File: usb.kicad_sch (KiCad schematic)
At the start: 5 parts, among them J13 USB-C 2.0, U9 USBLC6-2SC6

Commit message: friday changes
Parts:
- D7: DigiKey (none) -> 1655-DSS14UTR-ND
- J13: DigiKey (none) -> 2073-USB4085-GF-ATR-ND
- R15, R16: DigiKey (none) -> RMCF1206JT5K10TR-ND; MPN (none) -> RMCF1206JT5K10; Manufacturer (none) -> Stackpole Electronics Inc
- U9: DigiKey (none) -> 5399-USBLC6-2SC6TR-ND
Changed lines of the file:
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@@
+			)
+		)
+		(property "DigiKey" "2073-USB4085-GF-ATR-ND"
+			(at 0 0 0)
+			(effects
+				(font
+					(size 1.27 1.27)
+				)
+				(hide yes)
 			)
 		)
@@
 			)
 		)
+		(property "Manufacturer" "Stackpole Electronics Inc"
+			(at 0 0 0)
+			(effects
+				(font
+					(size 1.27 1.27)
+				)
+				(hide yes)
+			)
+		)
+		(property "MPN" "RMCF1206JT5K10"
+			(at 0 0 0)
+			(effects
+				(font
+					(size 1.27 1.27)
+				)
+				(hide yes)
+			)
+		)
+		(property "DigiKey" "RMCF1206JT5K10TR-ND"
+			(at 0 0 0)
+			(effects
+				(font
+					(size 1.27 1.27)
+				)
+				(hide yes)
+			)
+		)
 		(pin "1"
 		)
@@
 			)
 		)
+		(property "Manufacturer" "Stackpole Electronics Inc"
+			(at 0 0 0)
+			(effects
+				(font
+					(size 1.27 1.27)
+				)
+				(hide yes)
+			)
+		)
+		(property "MPN" "RMCF1206JT5K10"
+			(at 0 0 0)
+			(effects
+				(font
+					(size 1.27 1.27)
+				)
+				(hide yes)
+			)
+		)
+		(property "DigiKey" "RMCF1206JT5K10TR-ND"
+			(at 0 0 0)
+			(effects
+				(font
+					(size 1.27 1.27)
+				)
+				(hide yes)
+			)
+		)
 		(pin "1"
 		)
@@
 			)
 		)
+		(property "DigiKey" "1655-DSS14UTR-ND"
+			(at 0 0 0)
+			(effects
+				(font
+					(size 1.27 1.27)
+				)
+				(hide yes)
+			)
+		)
 		(pin "1"
 		)
@@
 				(hide yes)
 			)
+		)
+		(property "DigiKey" "5399-USBLC6-2SC6TR-ND"
+			(at 0 0 0)
+			(effects
+				(font
+					(size 1.27 1.27)
+				)
+				(hide yes)
+			)

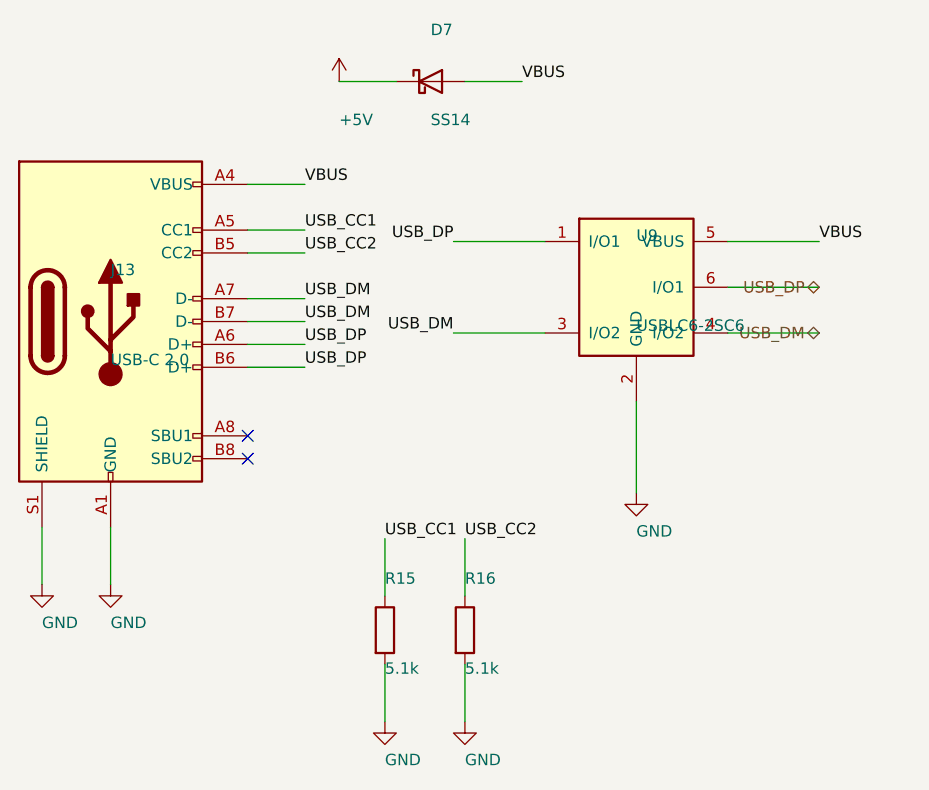
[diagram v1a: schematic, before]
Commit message: schematic updated
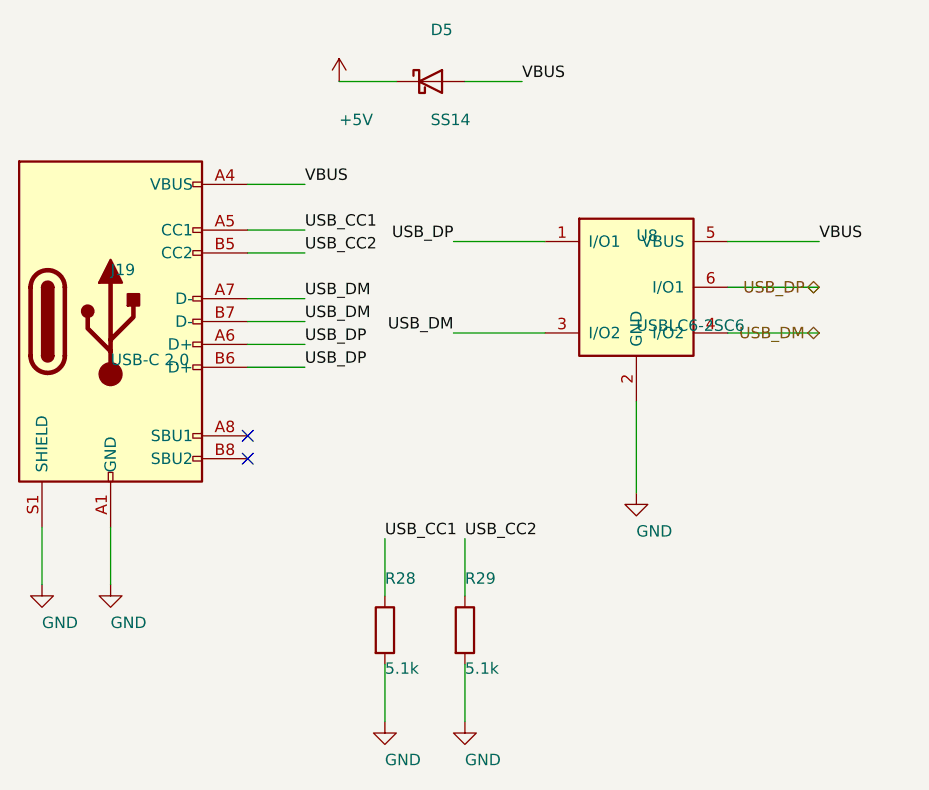
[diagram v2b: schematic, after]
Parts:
- renumbered D7 to D5, J13 to J19, R15 to R28, R16 to R29, U9 to U8
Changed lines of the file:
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@@
 		(on_board yes)
 		(dnp no)
-		(property "Reference" "J13"
+		(property "Reference" "J19"
 			(at 172.72 143.59 0)
 			(effects
@@
 			(project "controlcarreta"
 				(path "/9232987b-e923-413e-abd9-77ced6cc4c47/a9f5f58e-9f19-4b76-92d3-0178cc2d2479"
-					(reference "J13")
+					(reference "J19")
 					(unit 1)
 				)
@@
 		(on_board yes)
 		(dnp no)
-		(property "Reference" "#PWR0522"
+		(property "Reference" "#PWR0156"
 			(at 172.72 172.8 0)
 			(effects
@@
 			(project "controlcarreta"
 				(path "/9232987b-e923-413e-abd9-77ced6cc4c47/a9f5f58e-9f19-4b76-92d3-0178cc2d2479"
-					(reference "#PWR0522")
+					(reference "#PWR0156")
 					(unit 1)
 				)
@@
 		(on_board yes)
 		(dnp no)
-		(property "Reference" "#PWR0523"
+		(property "Reference" "#PWR0155"
 			(at 165.1 172.8 0)
 			(effects
@@
 			(project "controlcarreta"
 				(path "/9232987b-e923-413e-abd9-77ced6cc4c47/a9f5f58e-9f19-4b76-92d3-0178cc2d2479"
-					(reference "#PWR0523")
+					(reference "#PWR0155")
 					(unit 1)
 				)
@@
 		(on_board yes)
 		(dnp no)
-		(property "Reference" "R15"
+		(property "Reference" "R28"
 			(at 203.2 177.88 0)
 			(effects
@@
 			(project "controlcarreta"
 				(path "/9232987b-e923-413e-abd9-77ced6cc4c47/a9f5f58e-9f19-4b76-92d3-0178cc2d2479"
-					(reference "R15")
+					(reference "R28")
 					(unit 1)
 				)
@@
 		(on_board yes)
 		(dnp no)
-		(property "Reference" "#PWR0524"
+		(property "Reference" "#PWR0158"
 			(at 203.2 188.04 0)
 			(effects
@@
 			(project "controlcarreta"
 				(path "/9232987b-e923-413e-abd9-77ced6cc4c47/a9f5f58e-9f19-4b76-92d3-0178cc2d2479"
-					(reference "#PWR0524")
+					(reference "#PWR0158")
 					(unit 1)
 				)
@@
 		(on_board yes)
 		(dnp no)
-		(property "Reference" "R16"
+		(property "Reference" "R29"
 			(at 212.09 177.88 0)
 			(effects
@@
 			(project "controlcarreta"
 				(path "/9232987b-e923-413e-abd9-77ced6cc4c47/a9f5f58e-9f19-4b76-92d3-0178cc2d2479"
-					(reference "R16")
+					(reference "R29")
 					(unit 1)
 				)
@@
 		(on_board yes)
 		(dnp no)
-		(property "Reference" "#PWR0525"
+		(property "Reference" "#PWR0159"
 			(at 212.09 188.04 0)
 			(effects
@@
 			(project "controlcarreta"
 				(path "/9232987b-e923-413e-abd9-77ced6cc4c47/a9f5f58e-9f19-4b76-92d3-0178cc2d2479"
-					(reference "#PWR0525")
+					(reference "#PWR0159")
 					(unit 1)
 				)
@@
 		(on_board yes)
 		(dnp no)
-		(property "Reference" "D7"
+		(property "Reference" "D5"
 			(at 208.28 116.92 0)
 			(effects
@@
 			(project "controlcarreta"
 				(path "/9232987b-e923-413e-abd9-77ced6cc4c47/a9f5f58e-9f19-4b76-92d3-0178cc2d2479"
-					(reference "D7")
+					(reference "D5")
 					(unit 1)
 				)
@@
 		(on_board yes)
 		(dnp no)
-		(property "Reference" "#PWR0526"
+		(property "Reference" "#PWR0157"
 			(at 198.12 116.92 0)
 			(effects
@@
 			(project "controlcarreta"
 				(path "/9232987b-e923-413e-abd9-77ced6cc4c47/a9f5f58e-9f19-4b76-92d3-0178cc2d2479"
-					(reference "#PWR0526")
+					(reference "#PWR0157")
 					(unit 1)
 				)
@@
 		(on_board yes)
 		(dnp no)
-		(property "Reference" "U9"
+		(property "Reference" "U8"
 			(at 231.14 139.78 0)
 			(effects
@@
 			(project "controlcarreta"
 				(path "/9232987b-e923-413e-abd9-77ced6cc4c47/a9f5f58e-9f19-4b76-92d3-0178cc2d2479"
-					(reference "U9")
+					(reference "U8")
 					(unit 1)
 				)
@@
 		(on_board yes)
 		(dnp no)
-		(property "Reference" "#PWR0527"
+		(property "Reference" "#PWR0160"
 			(at 231.14 162.64 0)
 			(effects
@@
 			(project "controlcarreta"
 				(path "/9232987b-e923-413e-abd9-77ced6cc4c47/a9f5f58e-9f19-4b76-92d3-0178cc2d2479"
-					(reference "#PWR0527")
-					(unit 1)
-				)
+					(reference "#PWR0160")
+					(unit 1)
+				)

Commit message: last changes in work
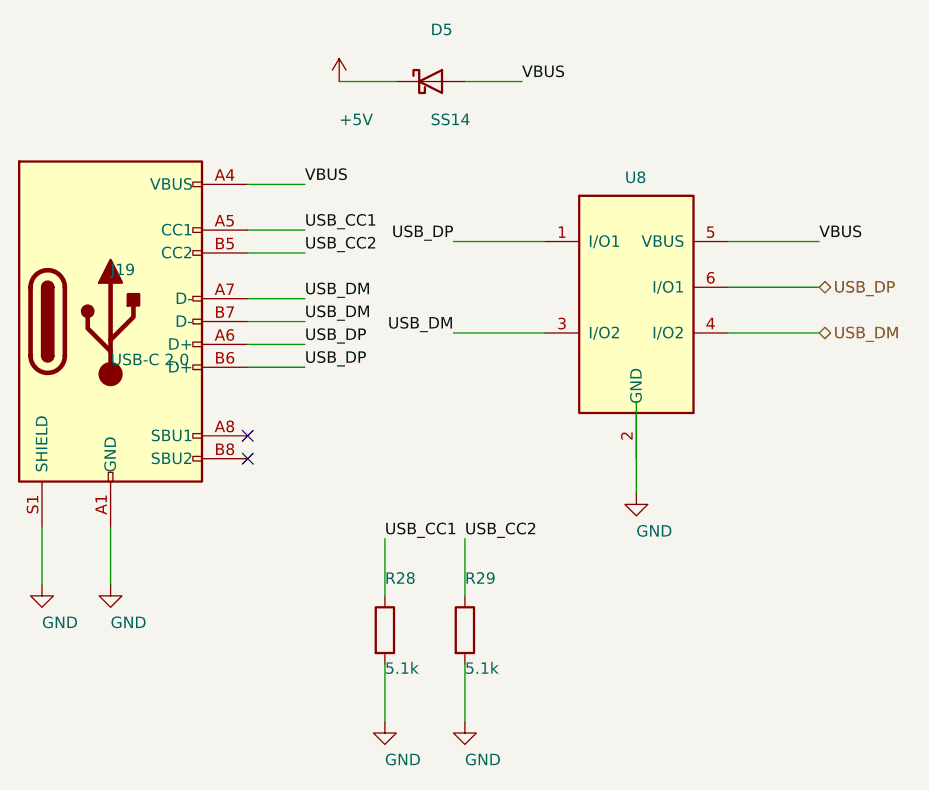
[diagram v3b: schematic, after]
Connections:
- net GND: no longer U8.2 (GND)
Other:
- moved on the sheet: U8
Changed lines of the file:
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@@
 	(hierarchical_label "USB_DP"
 		(shape bidirectional)
-		(at 251.46 144.78 180)
+		(at 251.46 144.78 0)
 		(effects
 			(font
 				(size 1.27 1.27)
 			)
-			(justify right)
+			(justify left)
 		)
 	)
 	(hierarchical_label "USB_DM"
 		(shape bidirectional)
-		(at 251.46 149.86 180)
+		(at 251.46 149.86 0)
 		(effects
 			(font
 				(size 1.27 1.27)
 			)
-			(justify right)
+			(justify left)
 		)
 	)
@@
 		(dnp no)
 		(property "Reference" "U8"
-			(at 231.14 139.78 0)
+			(at 229.87 133.35 0)
 			(effects
 				(font
@@
 		)
 		(property "Value" "USBLC6-2SC6"
-			(at 231.14 149.78 0)
-			(effects
-				(font
-					(size 1.27 1.27)
-				)
-				(justify left bottom)
+			(at 240.03 159.766 0)
+			(effects
+				(font
+					(size 1.27 1.27)
+				)
+				(justify left bottom)
+				(hide yes)
 			)
 		)
@@
 			)
 		)
-		(property "Datasheet" "https://www.digikey.com/en/products/detail/stmicroelectronics/USBLC6-2SC6/1121688"
+		(property "Datasheet" "https://www.digikey.com/en/products/detail/stmicroelectronics/USBLC6-2SC6/1040559"
 			(at 231.14 144.78 0)
 			(effects
